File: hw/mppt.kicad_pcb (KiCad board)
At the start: 4 copper layers, 100.1 x 55.1 mm, 361 parts, among them J201 1935776, J301 1935776, J302 1935776, Q301 SW_L, Q302 SW_H, SW201 SW_Push, U201 MCU_Nucleo_L432KC, U401 INA210, U402 INA210, U403 OPA990, U404 OPA990, U501 LMG1210RVRT

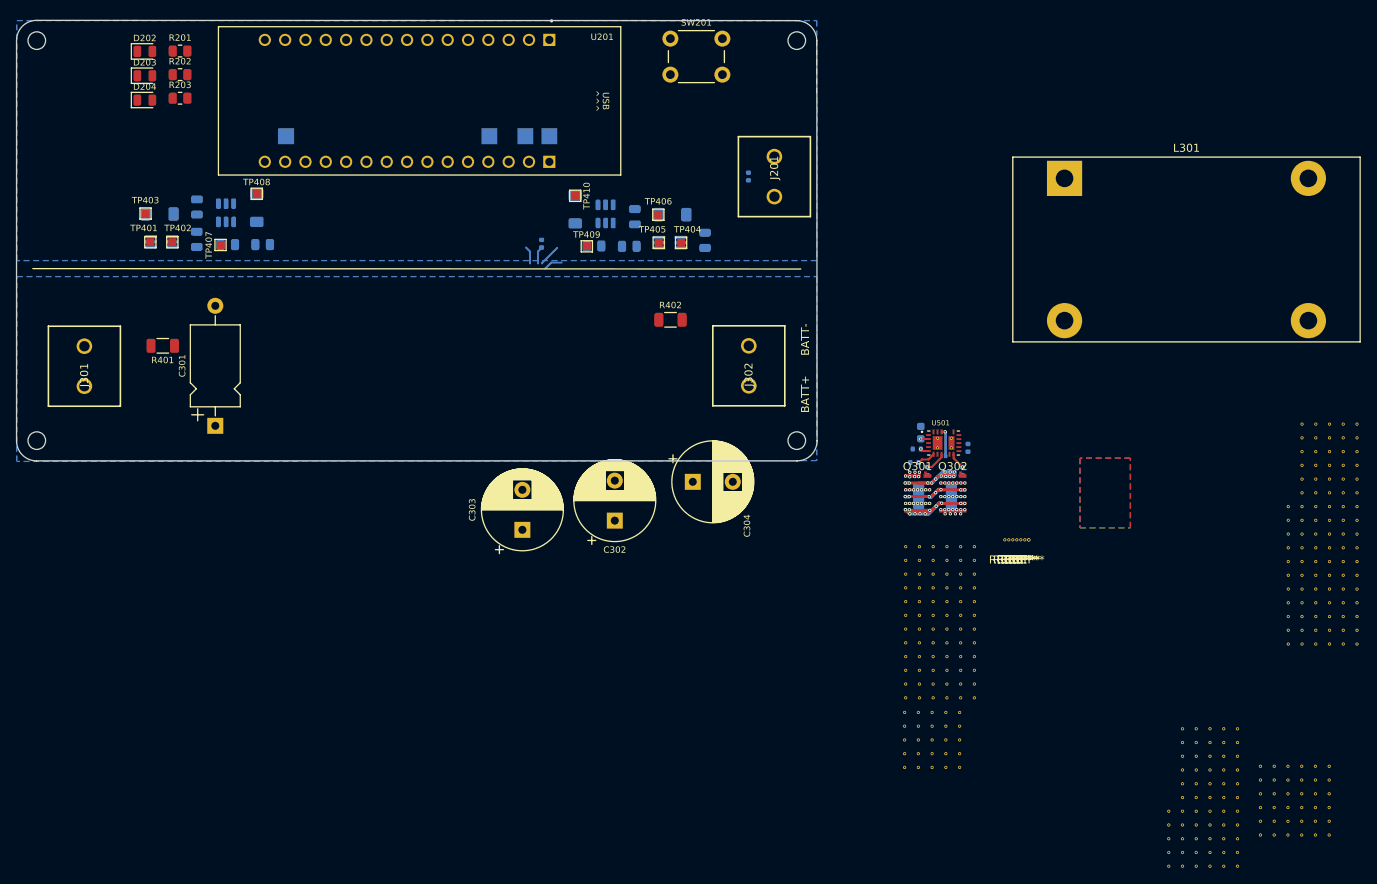
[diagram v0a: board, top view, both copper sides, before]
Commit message: layout revision this one is cursed
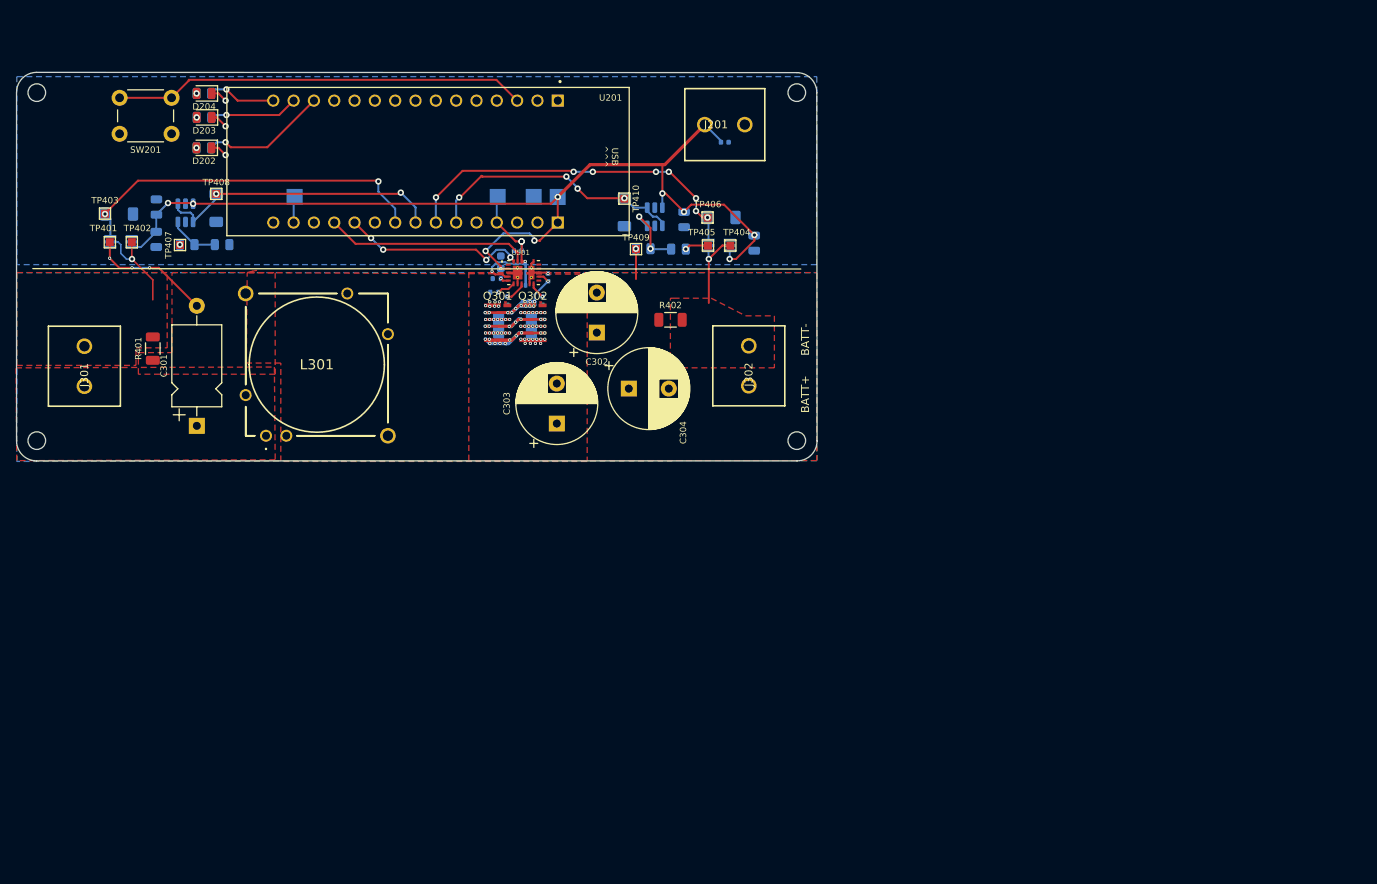
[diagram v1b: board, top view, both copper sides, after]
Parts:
- removed REF** (x7): Via_0.4mmOD_0.2mmID, mppt:Via_0.4mmOD_0.2mmID
- removed V1, V10, V100, V101, V102, V103, V104, V105, V106, V107, V108, V109, V11, V110, V111, V112, V113, V114, V115, V116, V117, V118, V119, V12, V120, V121, V122, V123, V124, V125, V126, V127, V128, V129, V13, V130, V131, V132, V133, V134, V135, V136, V137, V138, V139, V14, V140, V141, V142, V143, V144, V145, V146, V147, V148, V149, V15, V150, V151, V152, V153, V154, V155, V156, V157, V158, V159, V16, V160, V161, V162, V163, V164, V165, V166, V167, V168, V169, V17, V170, V171, V172, V173, V174, V175, V176, V177, V178, V179, V18, V180, V181, V182, V183, V184, V185, V186, V187, V188, V189, V19, V190, V191, V192, V193, V194, V195, V196, V197, V198, V199, V2, V20, V200, V201, V202, V203, V204, V205, V206, V207, V208, V209, V21, V210, V211, V212, V213, V214, V215, V216, V217, V218, V219, V22, V220, V221, V222, V223, V224, V225, V226, V227, V228, V229, V23, V230, V231, V232, V233, V234, V235, V236, V237, V238, V239, V24, V240, V241, V242, V243, V244, V245, V246, V247, V248, V249, V25, V250, V251, V252, V253, V254, V255, V256, V257, V258, V259, V26, V260, V261, V262, V263, V264, V265, V266, V267, V268, V269, V27, V270, V271, V272, V273, V274, V275, V276, V277, V278, V279, V28, V280, V281, V282, V283, V284, V285, V286, V287, V288, V289, V29, V3, V30, V31, V32, V33, V34, V35, V36, V37, V38, V39, V4, V40, V41, V42, V43, V44, V45, V46, V47, V48, V49, V5, V50, V51, V52, V53, V54, V55, V56, V57, V58, V59, V6, V60, V61, V62, V63, V64, V65, V66, V67, V68, V69, V7, V70, V71, V72, V73, V74, V75, V76, V77, V78, V79, V8, V80, V81, V82, V83, V84, V85, V86, V87, V88, V89, V9, V90, V91, V92, V93, V94, V95, V96, V97, V98, V99: 0.4mmVia, mppt:Via_0.4mmOD_0.2mmID
- L301: value 1529uH -> 560; footprint Inductor_THT:L_CommonMode_Toroid_Vertical_L43.2mm_W22.9mm_Px17.78mm_Py30.48mm_Bourns_8100 -> mppt:B65812N1005D002
- R201, R202, R203: moved to B.Cu
- moved L301 104.9 mm to (121.2, 111.9)
- moved SW201 63.5 mm to (109.3, 74.2), turned to 180 degrees
- moved C1 56.7 mm to (152.3, 98.1)
- moved C503 56.7 mm to (156.4, 92.1)
- moved C502 56.7 mm to (150.5, 90.2)
- moved D1 56.7 mm to (153.6, 94.2)
- moved Q301 56.7 mm to (150.1, 97.6)
- moved Q302 56.7 mm to (154.5, 97.6)
- moved R501 56.7 mm to (149.7, 94.0)
- moved R502 56.7 mm to (150.0, 92.2)
- moved R503 56.7 mm to (151.3, 95.0)
- moved R504 56.7 mm to (155.7, 95.0)
- moved U501 56.7 mm to (153.3, 91.5)
- moved C302 23.6 mm to (162.5, 99.0)
- moved D202 14.1 mm to (113.4, 75.9), turned to 180 degrees
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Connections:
- net V_SW renamed /converter/V_SW
- D1 pad 2: /gate_driver/BST -> +5V
- U501 pad 17: /gate_driver/BST -> +5V
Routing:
- net +12V: track 3.14 -> 126.6 mm, vias 1 -> 10
- net /controller/Reset: track 0.00 -> 51.8 mm
- net /controller/ARR_CURRENT: track 0.00 -> 45.1 mm, vias 0 -> 2
- net /controller/BATT_CURRENT: track 0.00 -> 44.7 mm, vias 0 -> 8
- net /controller/ARR_VOLTAGE: track 0.00 -> 36.6 mm, vias 0 -> 2
- net /controller/BATT_VOLTAGE: track 0.00 -> 33.0 mm, vias 0 -> 4
- net GND: track 0.00 -> 26.7 mm, vias 21 -> 28
- net /controller/PWM_EN: track 0.00 -> 25.6 mm
- net /converter/V_ARR+: track 0.00 -> 23.6 mm, vias 0 -> 1
- net /controller/PWM: track 0.00 -> 23.2 mm, vias 0 -> 4
- net +5V: track 2.19 -> 21.7 mm, vias 0 -> 4
- net /controller/Heartbeat: track 0.00 -> 15.8 mm, vias 0 -> 1
- net /converter/V_ARR-: track 0.00 -> 12.5 mm, vias 0 -> 1
- net /controller/Tracking: track 0.00 -> 11.3 mm, vias 0 -> 1
- net /converter/V_BATT-: track 0.00 -> 9.94 mm, vias 0 -> 1
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- added copper zone on F.Cu, net /converter/V_ARR+
- added copper zone on F.Cu, net /converter/V_ARR-
- added copper zone on In1.Cu, net /converter/V_ARR-
- added copper zone on F.Cu, net /converter/V_BATT-
- added copper zone on In1.Cu, net /converter/V_BATT-
- added copper zone on F.Cu, net GND
- removed copper zone on B.Cu, net /converter/V_BATT+
- removed copper zone on In1.Cu, net /converter/V_BATT+
- removed copper zone on In2.Cu, net /converter/V_BATT+
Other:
- board size 100.1 x 55.1 mm -> 100.1 x 48.6 mm
- board text added: "INCOMPLETE"
- board text added: "LAYOUT WILL BE REVISED SIGNIFICANTLY"
- board text added: "PENDING"
